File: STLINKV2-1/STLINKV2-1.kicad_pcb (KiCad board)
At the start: 2 copper layers, 52.3 x 25.4 mm, 47 parts, among them J1 USB_A, J2 Conn_01x04, J3 Top, J4 Buttom, J5 Conn_01x02, Q1 MMBT5551L, U1 TLV73333PDBV, U2 STM32F103C8Tx, Y1 8M

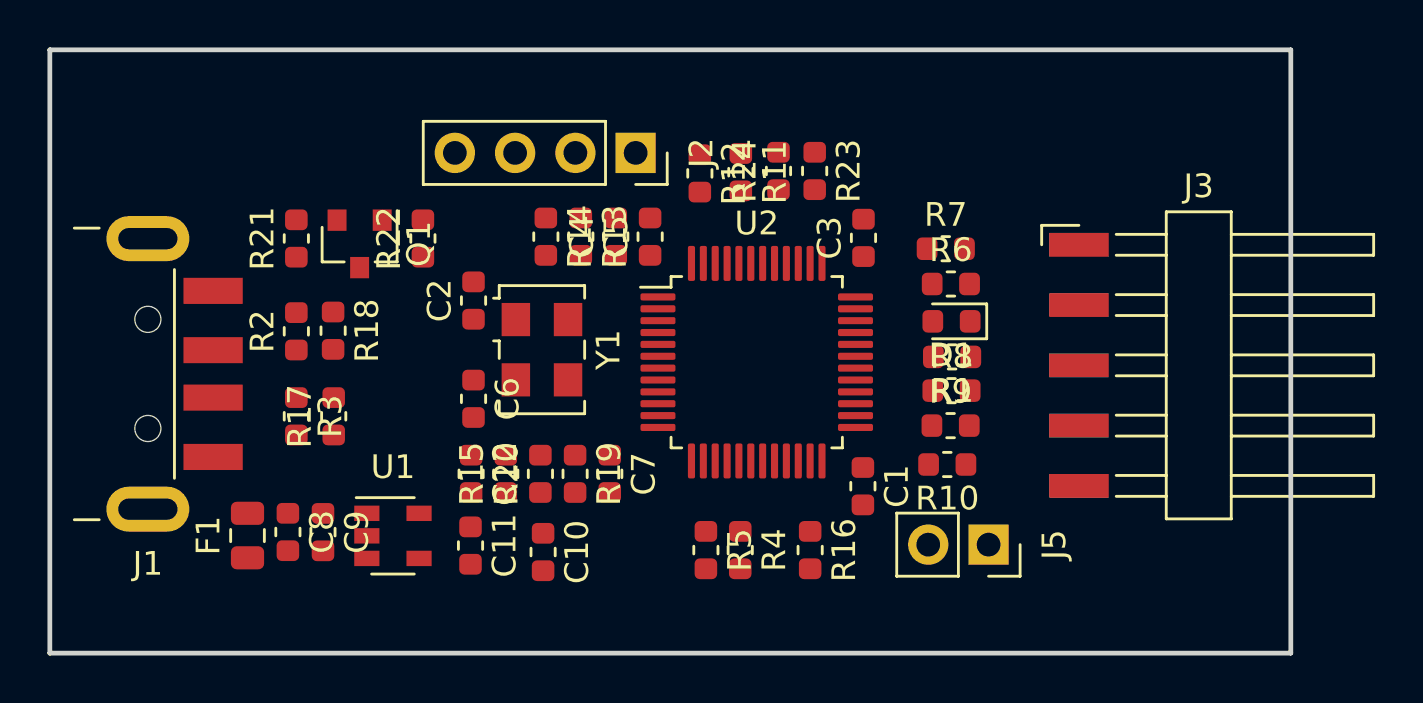
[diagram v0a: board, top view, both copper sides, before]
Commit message: layout finished
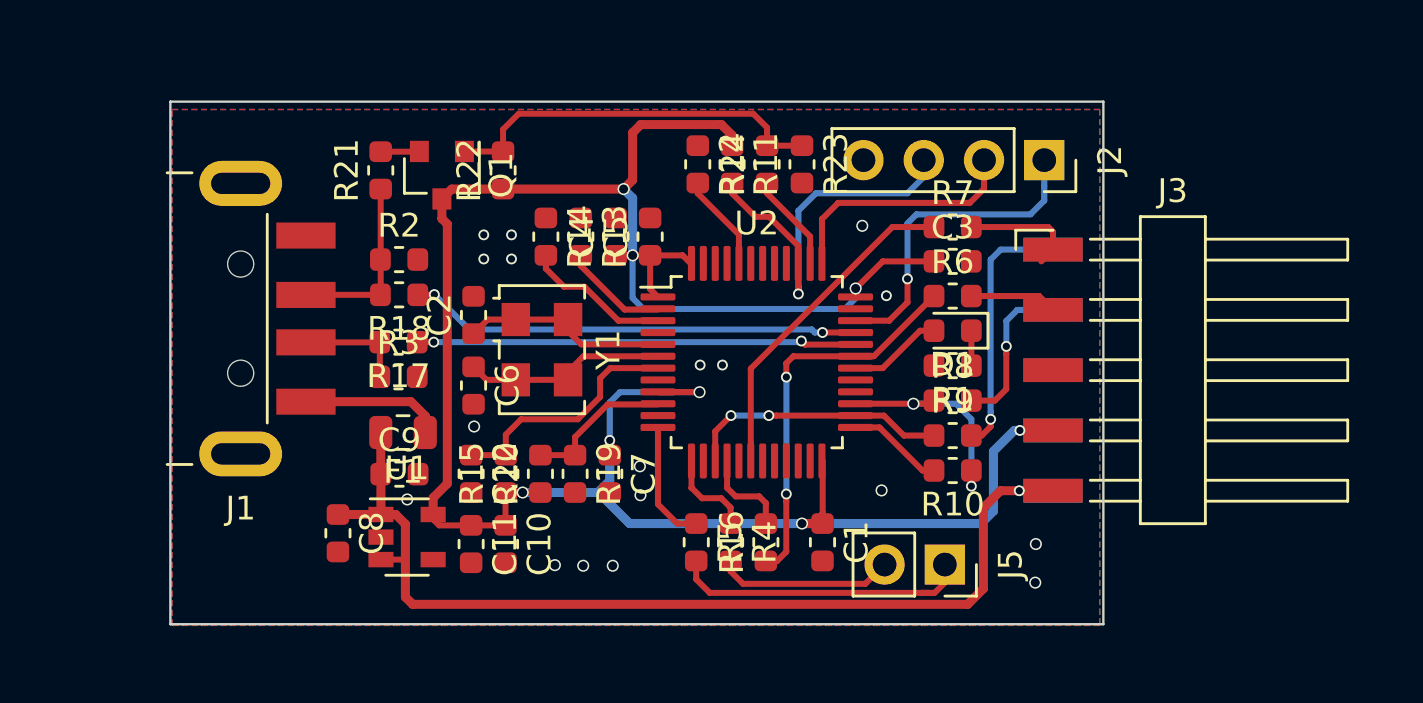
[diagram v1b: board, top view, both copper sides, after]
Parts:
- moved J2 17.2 mm to (130.8, 106.2)
- moved F1 7.86 mm to (103.8, 117.7), turned to 180 degrees
- moved R2 5.28 mm to (103.6, 110.4), turned to 0 degrees
- moved R3 4.62 mm to (103.6, 115.4), turned to 0 degrees
- moved R21 4.57 mm to (102.8, 106.7)
- moved J1 4.55 mm to (90.0, 112.9)
- moved Q1 4.52 mm to (105.4, 106.9)
- moved R22 4.43 mm to (108.0, 106.7)
- moved R17 4.15 mm to (103.6, 113.9), turned to 180 degrees
- moved C9 4.04 mm to (103.6, 119.5), turned to 0 degrees
- moved C3 3.89 mm to (126.9, 110.5), turned to 0 degrees
- moved R18 3.17 mm to (103.6, 111.9), turned to 180 degrees
- moved C1 2.91 mm to (121.5, 122.3)
- moved C8 2.11 mm to (101.0, 121.9)
- moved J5 2.02 mm to (126.6, 123.3)
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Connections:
- Y1 pad 3: (no net) -> /OSC_OUT
- Y1 pad 4: (no net) -> /OSC_IN
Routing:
- net +3V3: track 0.00 -> 102.5 mm, vias 0 -> 8
- net +5V: track 0.00 -> 42.0 mm, vias 0 -> 1
- net /USB0_P: track 0.00 -> 19.1 mm, vias 0 -> 2
- net /USB0_N: track 0.00 -> 18.6 mm, vias 0 -> 2
- net /SWO0: track 0.00 -> 16.6 mm, vias 0 -> 1
- net Net-(Q1-Pad1): track 0.00 -> 16.4 mm
- net /T_SWO: track 0.00 -> 16.4 mm, vias 0 -> 2
- net /T_NRST: track 0.00 -> 14.1 mm
- net /SWDIO0: track 0.00 -> 13.7 mm, vias 0 -> 1
- net /P_TXD: track 0.00 -> 12.8 mm
- net /T_JTCK: track 0.00 -> 11.1 mm, vias 0 -> 2
- net /P_SWCLK: track 0.00 -> 10.8 mm, vias 0 -> 1
- net /SWCLK0: track 0.00 -> 10.4 mm
- net Net-(C12-Pad1): track 0.00 -> 10.4 mm
- net /T_JTMS: track 0.00 -> 9.50 mm, vias 0 -> 2
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- added copper zone on B.Cu, net GND
- added copper zone on F.Cu, net GND
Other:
- board size 52.3 x 25.4 mm -> 39.3 x 22 mm
- net class Default: clearance 0.00508 -> 0.127
- net class POWER: clearance 0.254 -> 0.127
- net class SIGNAL: clearance 0.00508 -> 0.127
- rule trace_clearance: 0.00508 -> 0.127
